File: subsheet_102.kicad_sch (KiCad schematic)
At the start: 14 parts, among them J7 MIDI IN, J8 MIDI OUT, U20 MC6850_PHY, U35 74LS04_PHY, U39 PC900_PHY

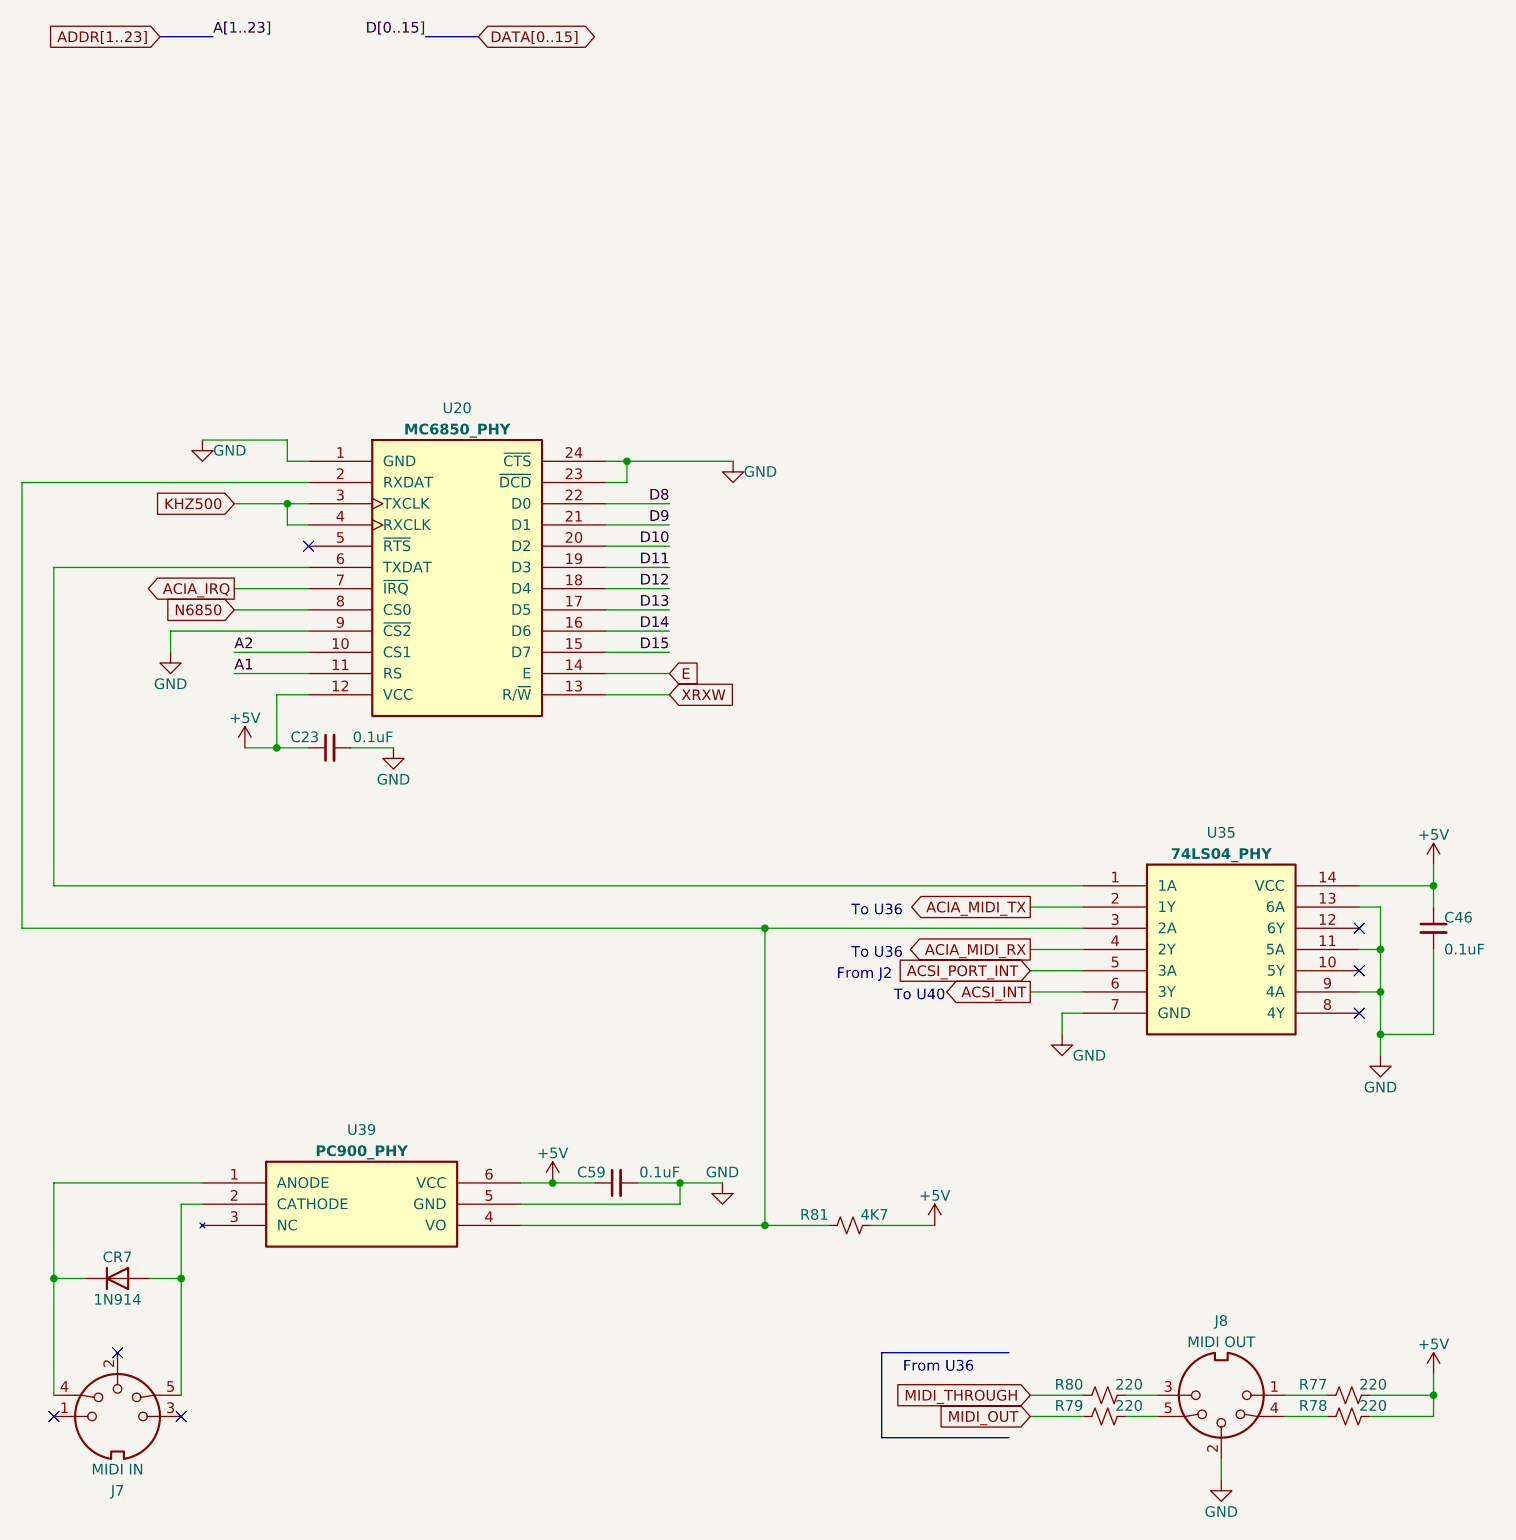
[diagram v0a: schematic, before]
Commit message: complete hsync to line_phase for modulator
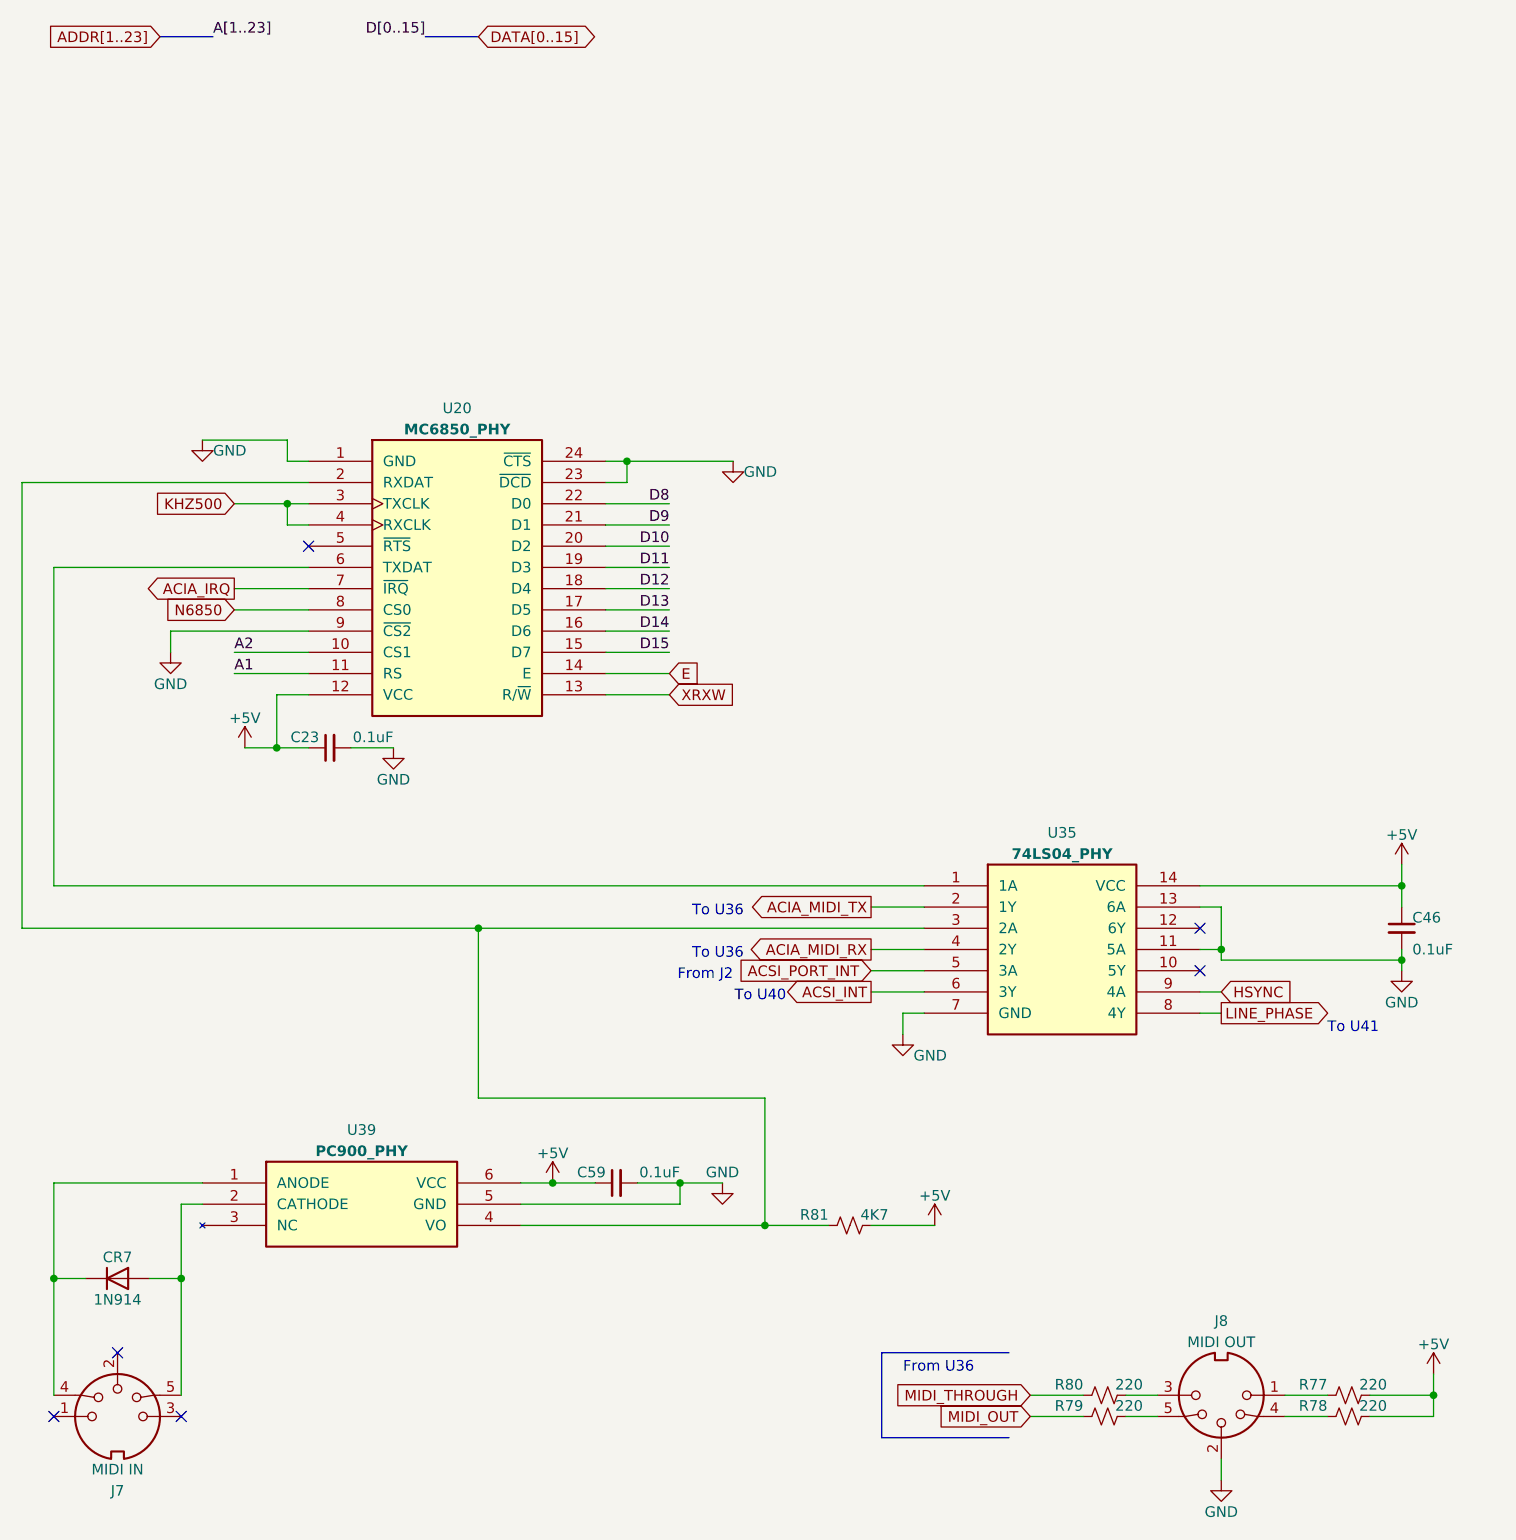
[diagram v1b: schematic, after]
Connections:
- net GND: no longer U35.9 (4A)
- net LINE_PHASE: now reaches U35.8 (4Y)
- new net HSYNC: U35.9 (4A)
- no-connect marks 7 -> 6
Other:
- note added: "To U41"
- moved on the sheet: C46, U35
